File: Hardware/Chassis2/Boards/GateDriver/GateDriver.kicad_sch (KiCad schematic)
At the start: 34 parts, among them J2 TBP01R2W-508-06BE, J3 TBP01R2W-508-06BE, J4 TBP01R2W-508-06BE, J5 Conn_02x10_Counter_Clockwise, U5 BTS462TATMA1, U6 BTS462TATMA1

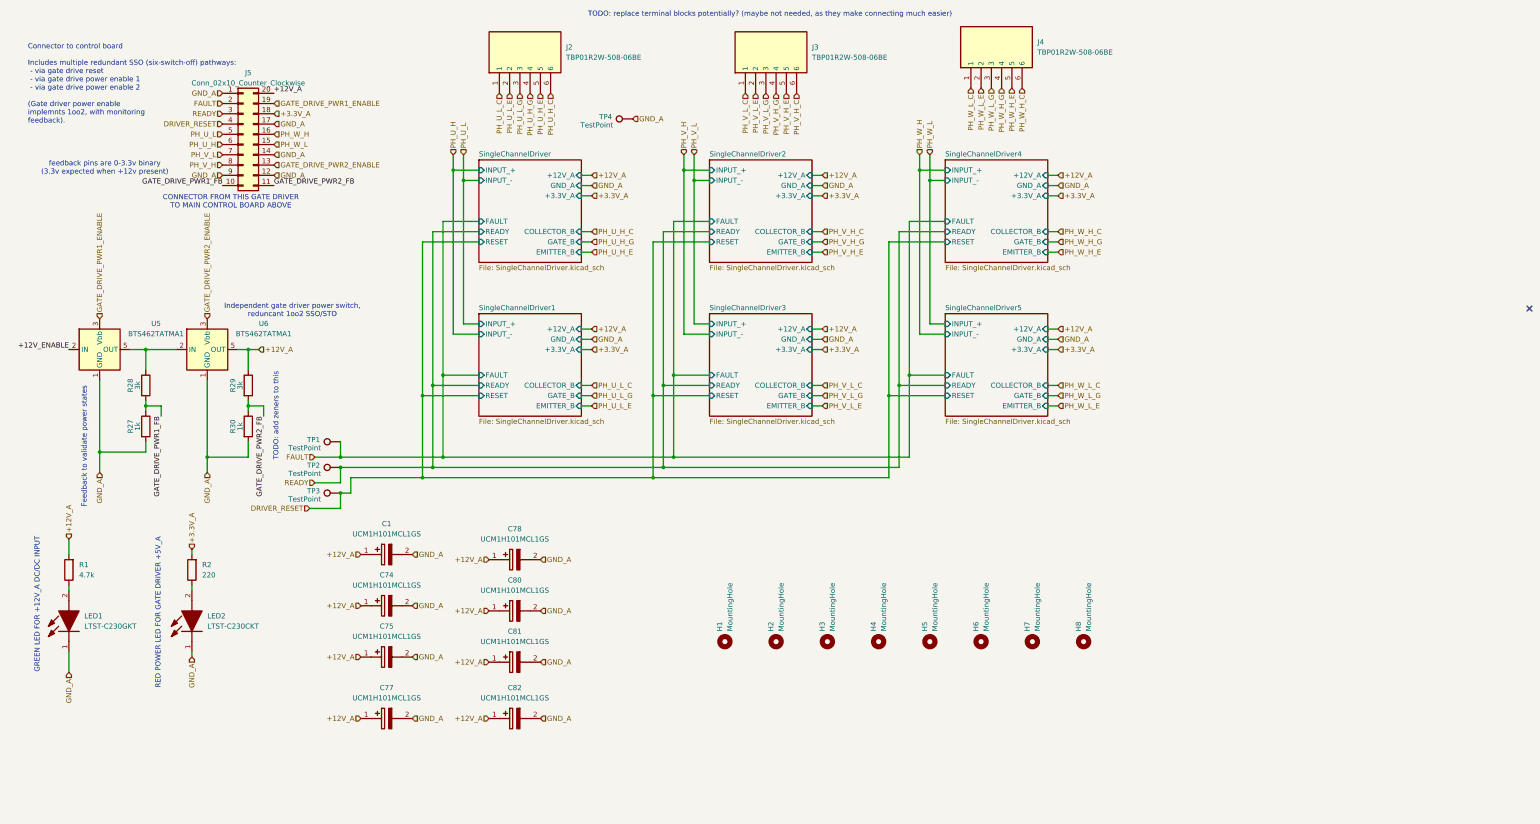
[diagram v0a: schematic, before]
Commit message: Update boards
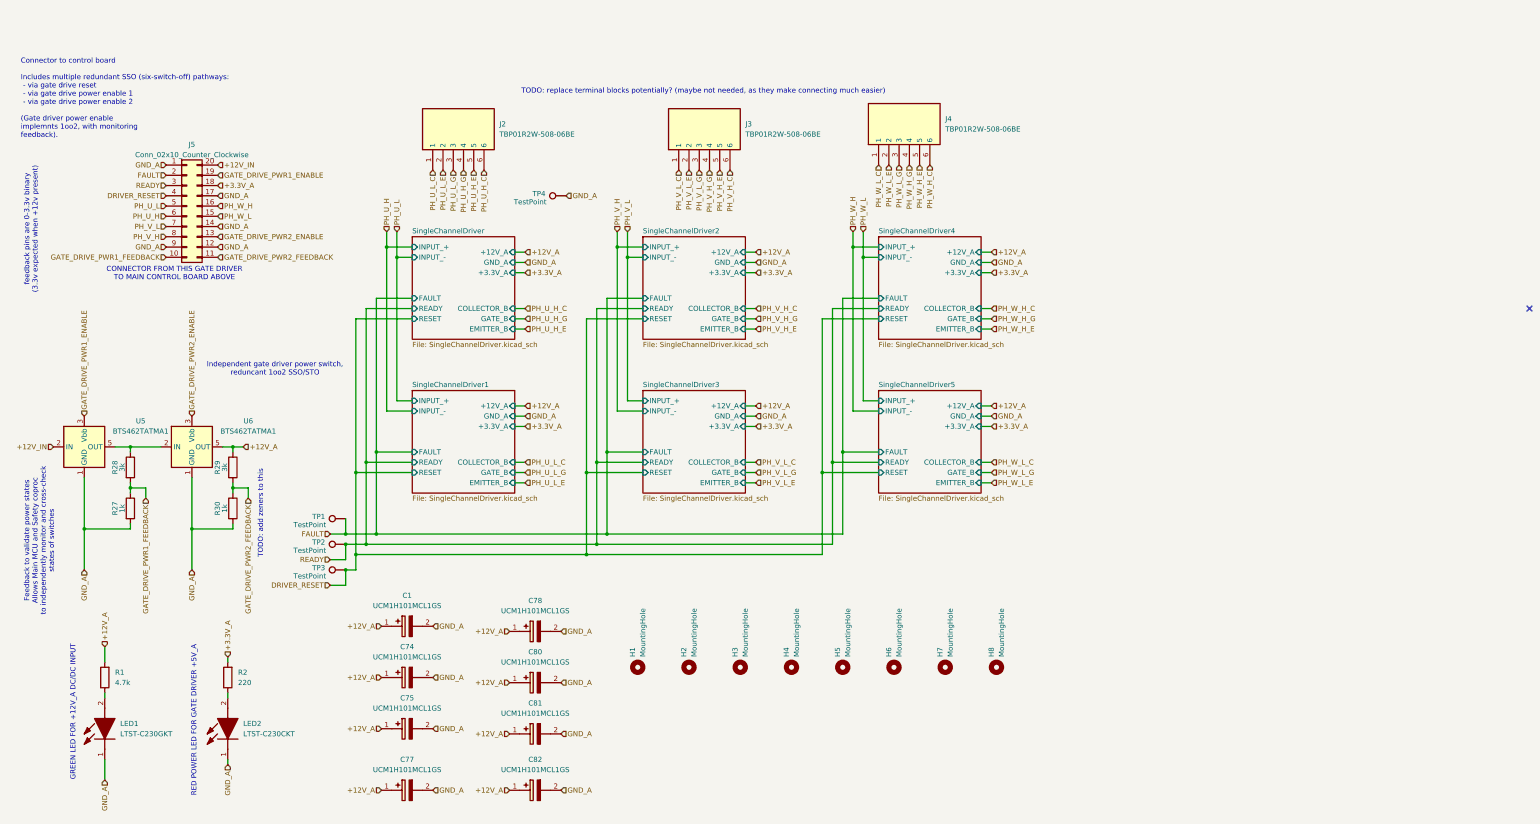
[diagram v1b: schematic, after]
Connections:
- net +12V_A: no longer J5.20 (Pin_20)
- net +12V_ENABLE renamed +12V_IN
- net +12V_IN: now also J5.20 (Pin_20)
- net GATE_DRIVE_PWR1_FB renamed GATE_DRIVE_PWR1_FEEDBACK
- net GATE_DRIVE_PWR2_FB renamed GATE_DRIVE_PWR2_FEEDBACK
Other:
- note added: "Feedback to validate power states Allows Main MCU and Safety coproc to independently monitor and cross-check states of switches"
- note removed: "Feedback to validate power states"
- moved on the sheet: C1, C74, C75, C77, C78, C80, C81, C82, H1, H2, H3, H4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

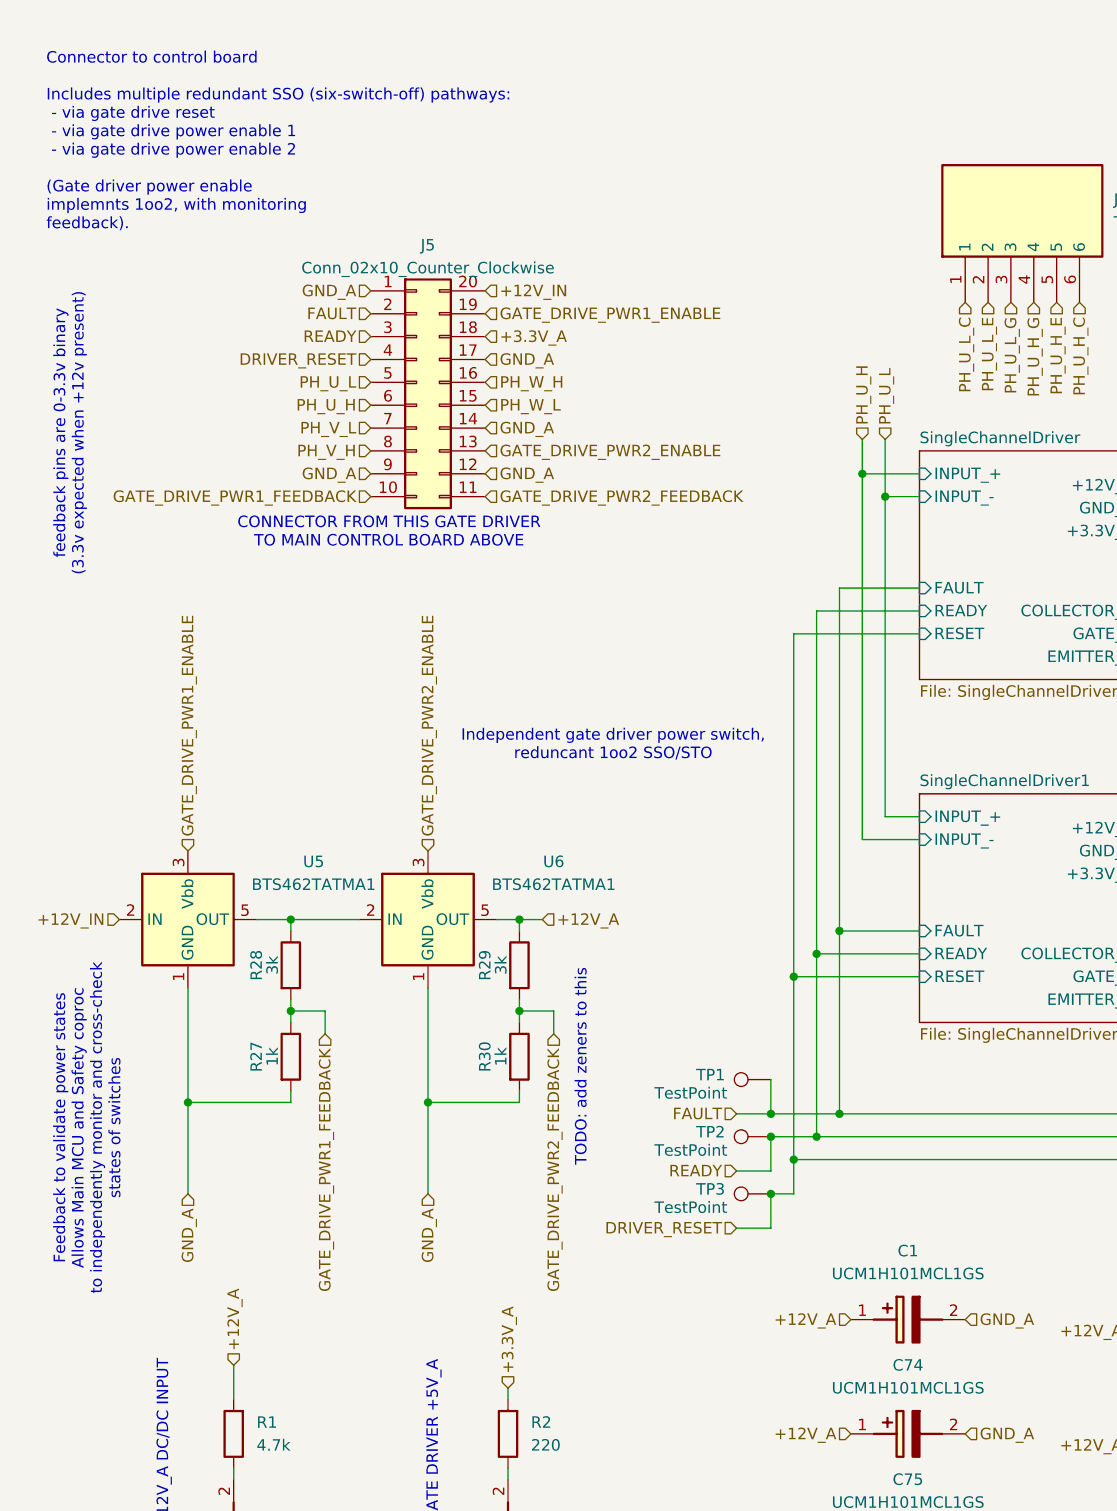
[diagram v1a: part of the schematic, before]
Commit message: eod 2026-07-08
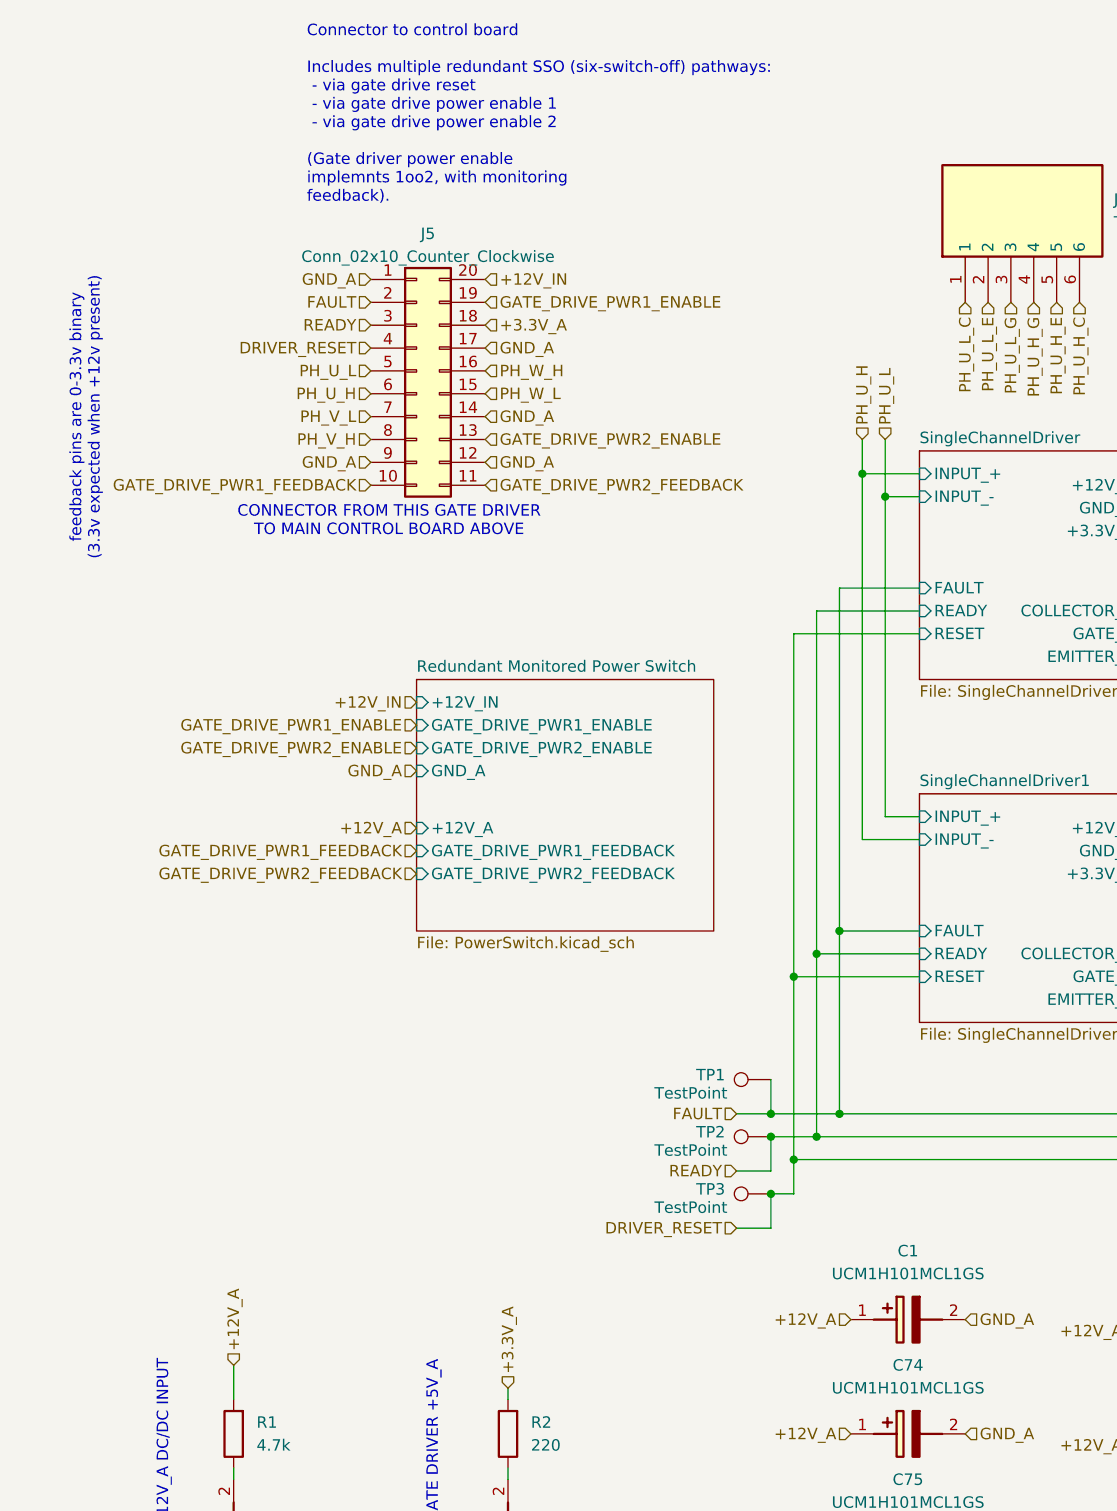
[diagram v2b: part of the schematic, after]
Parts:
- removed R27, R30: 1k, Resistor_SMD:R_1210_3225Metric_Pad1.30x2.65mm_HandSolder, symbol Device:R
- removed R28, R29: 3k, Resistor_SMD:R_1210_3225Metric_Pad1.30x2.65mm_HandSolder, symbol Device:R
- removed U5, U6: BTS462TATMA1, Package_TO_SOT_SMD:TO-252-4, symbol Power_Management:BTS462TATMA1
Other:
- added sheet Redundant Monitored Power Switch (PowerSwitch.kicad_sch)
- note removed: "Feedback to validate power states Allows Main MCU and Safety coproc to independently monitor and cross-check states of switches"
- note removed: "Independent gate driver power switch, reduncant 1oo2 SSO/STO"
- note removed: "TODO: add zeners to this"
- moved on the sheet: J5
